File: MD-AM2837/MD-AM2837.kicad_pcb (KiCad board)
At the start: 2 copper layers, 47 x 36 mm, 21 parts, among them J1 XT60_Male_Horizontal, J2 XT60_Female_Horizontal, J3 Conn_01x03_Pin_signal, Q1 BSS138, Q2 BSS138

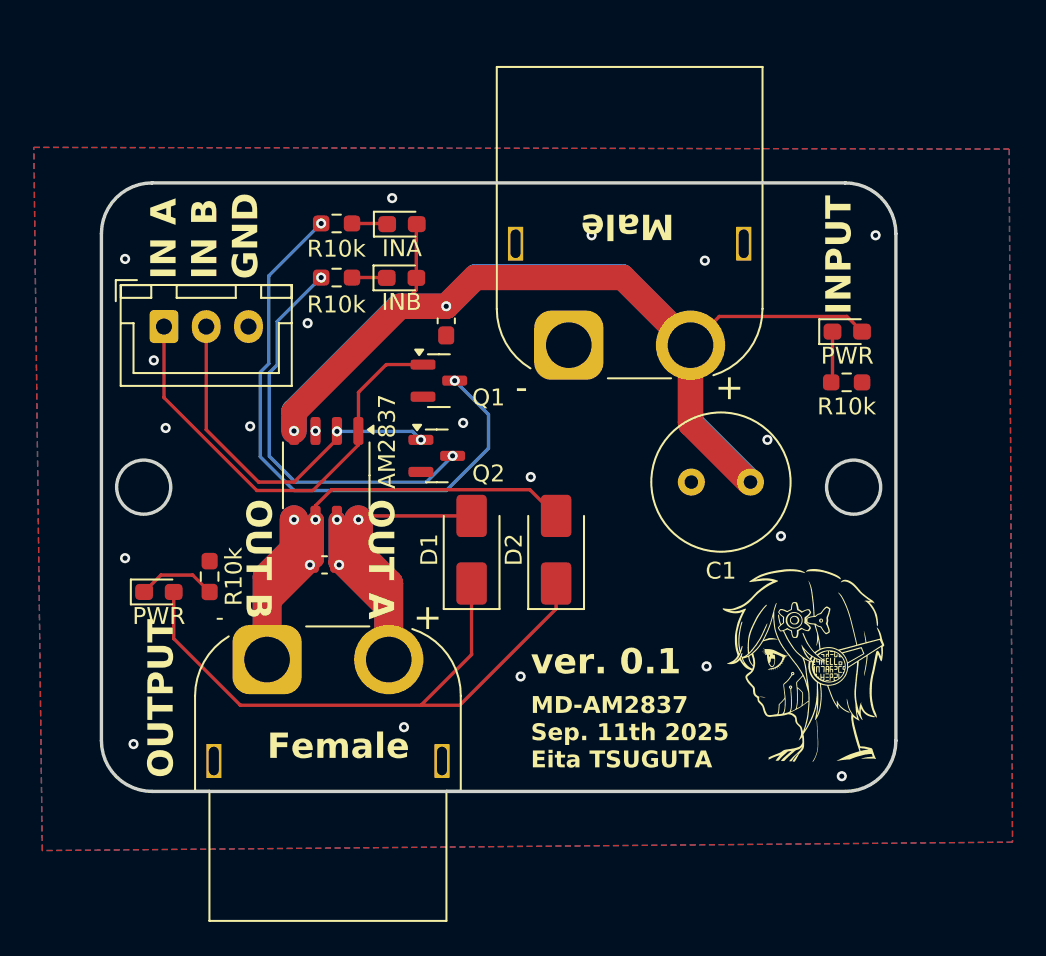
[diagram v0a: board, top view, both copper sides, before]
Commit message: v0.2作成
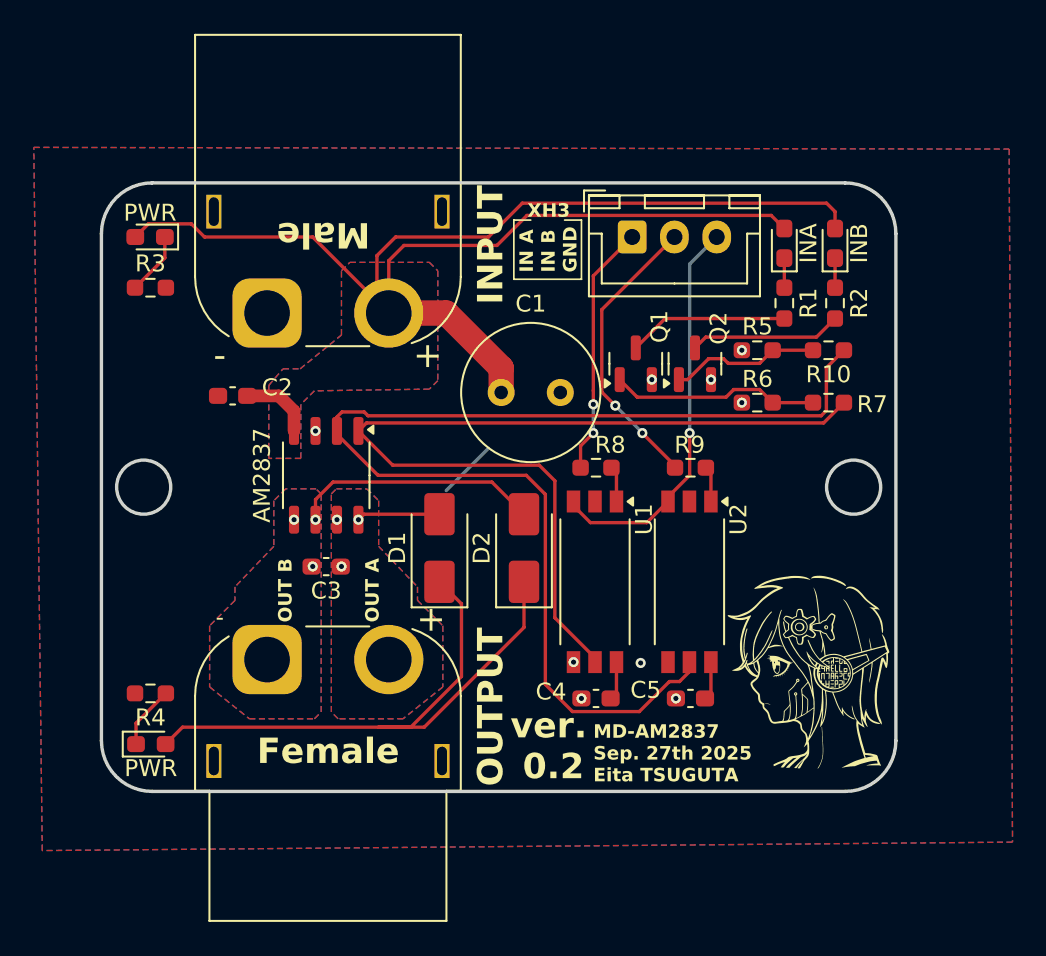
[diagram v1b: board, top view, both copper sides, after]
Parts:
- added C4: 0.1, Capacitor_SMD:C_0603_1608Metric_Pad1.08x0.95mm_HandSolder, F.Cu at (115.9, 93.3)
- added C5: 0.1, Capacitor_SMD:C_0603_1608Metric_Pad1.08x0.95mm_HandSolder, F.Cu at (121.4, 93.3)
- added R10: 1k, Resistor_SMD:R_0603_1608Metric_Pad0.98x0.95mm_HandSolder, F.Cu at (129.6, 72.7)
- added R5: 10k, Resistor_SMD:R_0603_1608Metric_Pad0.98x0.95mm_HandSolder, F.Cu at (125.4, 72.7)
- added R6: 10k, Resistor_SMD:R_0603_1608Metric_Pad0.98x0.95mm_HandSolder, F.Cu at (125.4, 75.8)
- added R7: 1k, Resistor_SMD:R_0603_1608Metric_Pad0.98x0.95mm_HandSolder, F.Cu at (129.6, 75.8)
- added R8: 10, Resistor_SMD:R_0603_1608Metric_Pad0.98x0.95mm_HandSolder, F.Cu at (115.9, 79.7)
- added R9: 10, Resistor_SMD:R_0603_1608Metric_Pad0.98x0.95mm_HandSolder, F.Cu at (121.4, 79.7)
- added U1: TLP2745, Package_SO:SO-6L_10x3.84mm_P1.27mm, F.Cu at (115.8, 86.4)
- added U2: TLP2745, Package_SO:SO-6L_10x3.84mm_P1.27mm, F.Cu at (121.4, 86.4)
- C1: value 220uF -> 220
- C2, C3: value 0.1uF -> 0.1
- R1, R2, R3, R4: value R10k -> 1k
- moved LED3 41.6 mm to (89.5, 66.0), turned to 180 degrees
- moved R3 41.6 mm to (89.5, 69.0)
- moved R2 29.5 mm to (130.0, 69.9), turned to -90 degrees
- moved J3 28.2 mm to (118.0, 66.0)
- moved R1 26.9 mm to (127.0, 69.9), turned to -90 degrees
- moved LED2 25.7 mm to (130.0, 66.4), turned to 90 degrees
- moved LED1 22.6 mm to (127.0, 66.4), turned to 90 degrees
- moved J1 18.0 mm to (96.4, 70.5)
- moved Q2 16.2 mm to (121.7, 73.5), turned to 90 degrees
- moved C1 15.7 mm to (110.2, 75.2), turned to 0 degrees
- moved C2 13.4 mm to (94.4, 75.4), turned to 0 degrees
- moved Q1 11.7 mm to (118.2, 73.5), turned to 90 degrees
- moved LED4 9.01 mm to (89.5, 96.0)
- moved R4 7.75 mm to (89.5, 93.0), turned to 180 degrees
- moved D1 1.90 mm to (106.6, 84.4)
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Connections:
- J3 pad 1: IN_A -> IN_A_1
- J3 pad 2: IN_B -> IN_B_1
- J3 pad 3: GND -> GNDS
- MD1 pad 1: IN_A -> IN_A_2
- MD1 pad 2: IN_B -> IN_B_2
- Q1 pad 1: IN_A -> Net-(Q1-G)
- Q2 pad 1: IN_B -> Net-(Q2-G)
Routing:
- net IN_B_2: track 0.00 -> 70.1 mm
- net IN_A_2: track 0.00 -> 54.0 mm
- net OUT_A: track 43.9 -> 4.93 mm
- net OUT_B: track 52.9 -> 14.7 mm
- net IN_A: track 26.7 -> 0.00 mm
- net Net-(Q1-D): track 35.5 -> 9.51 mm, vias 2 -> 0
- net GNDS: track 0.00 -> 23.6 mm, vias 0 -> 1
- net IN_B: track 21.8 -> 0.00 mm, vias 2 -> 0
- net IN_B_1: track 0.00 -> 17.2 mm, vias 0 -> 2
- net Net-(Q2-D): track 24.0 -> 9.01 mm, vias 2 -> 0
- net IN_A_1: track 0.00 -> 14.9 mm, vias 0 -> 2
- net Net-(Q1-G): track 0.00 -> 12.4 mm
- net Net-(Q2-G): track 0.00 -> 8.89 mm
- net GND: track 0.00 -> 3.54 mm, vias 20 -> 9
- net Vcc_U2: track 0.00 -> 2.29 mm
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- added copper zone on B.Cu, net OUT_A
- added copper zone on F.Cu, net OUT_A
- added copper zone on B.Cu, net OUT_B
- added copper zone on F.Cu, net OUT_B
- added copper zone on B.Cu, net VCC
- added copper zone on F.Cu, net VCC
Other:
- board text added: "MD-AM2837 Sep. 27th 2025 Eita TSUGUTA"
- board text added: "OUT B OUT A"
- board text added: "XH3"
- board text added: "ver. 0.2"
- board text removed: "MD-AM2837 Sep. 11th 2025 Eita TSUGUTA"
- board text removed: "OUT A OUT B"
- board text removed: "ver. 0.1"
